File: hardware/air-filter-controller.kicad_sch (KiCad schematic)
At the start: 64 parts, among them J1 TYPE-C-31-M-12, J13 Conn_01x02, J14 Conn_01x02, J2 Conn_01x05, J4 Conn_01x03, Q1 AO3400A, SW1 SW_Push, SW2 SW_Push, SW3 SW_Push, SW4 SW_Push, U1 ESP32-S3-WROOM-1-N4, U2 BMP280, U3 MT2492

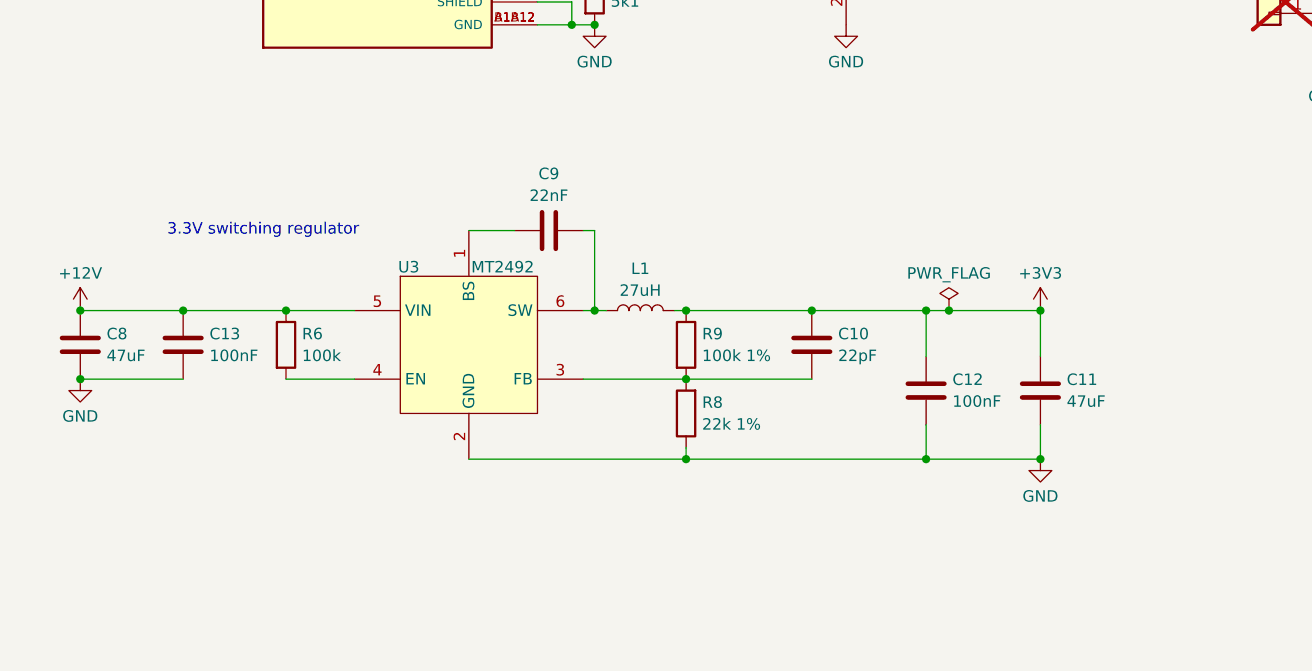
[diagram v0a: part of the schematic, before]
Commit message: Hardware v1.0
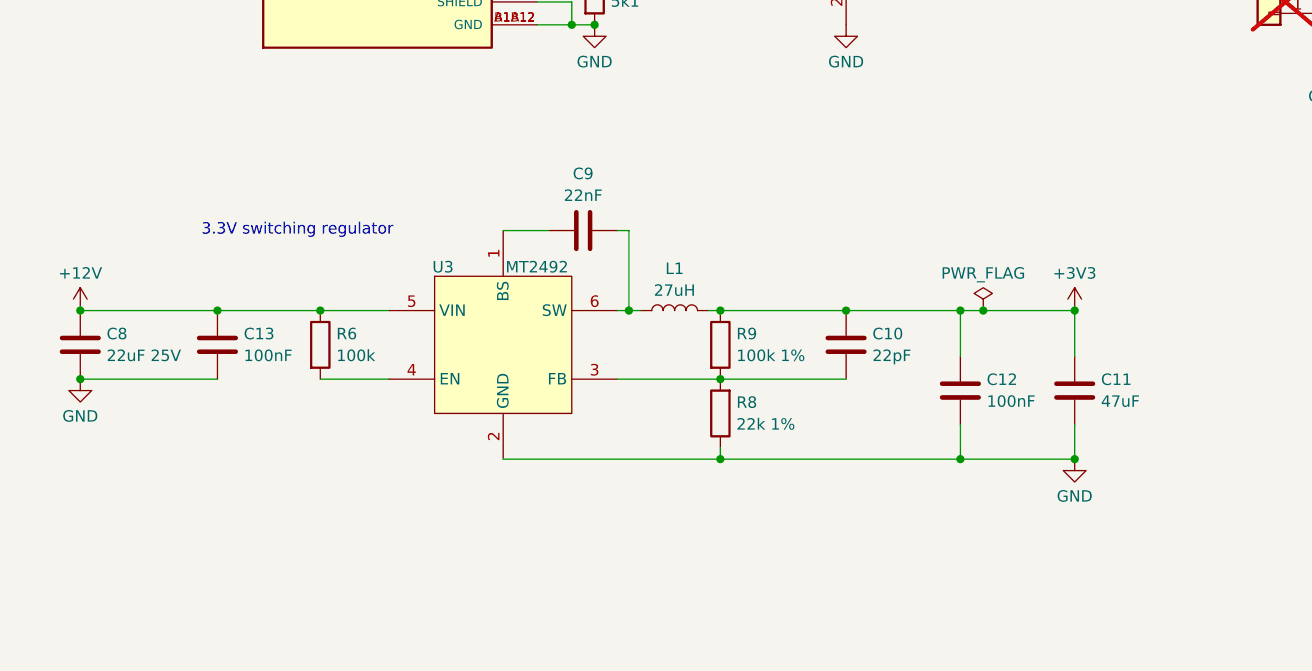
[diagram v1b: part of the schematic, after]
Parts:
- C8: value 47uF -> 22uF 25V; LCSC C96123 -> C12891
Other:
- moved on the sheet: C10, C11, C12, C13, C9, L1, R6, R8, R9, U3
